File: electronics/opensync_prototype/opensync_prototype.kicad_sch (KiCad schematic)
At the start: 0 parts

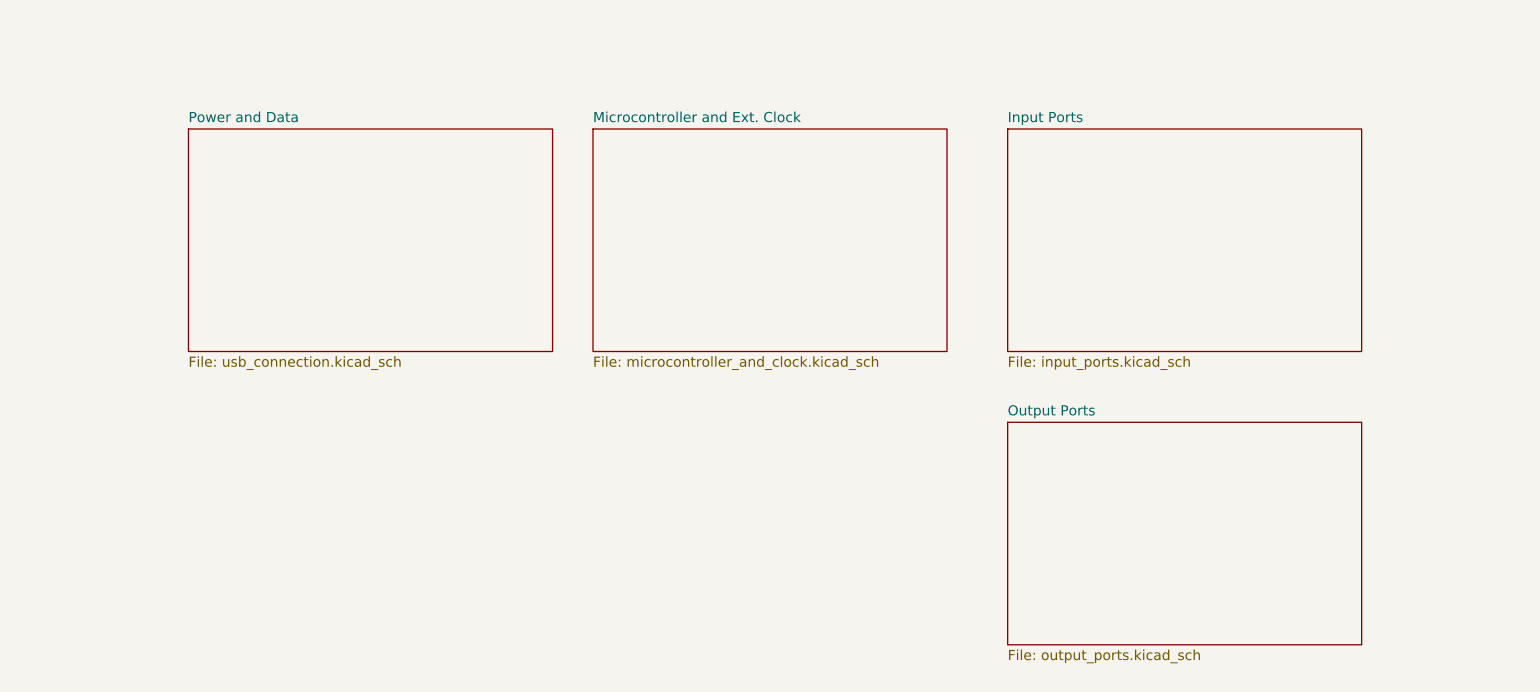
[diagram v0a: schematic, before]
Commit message: Emergency backup
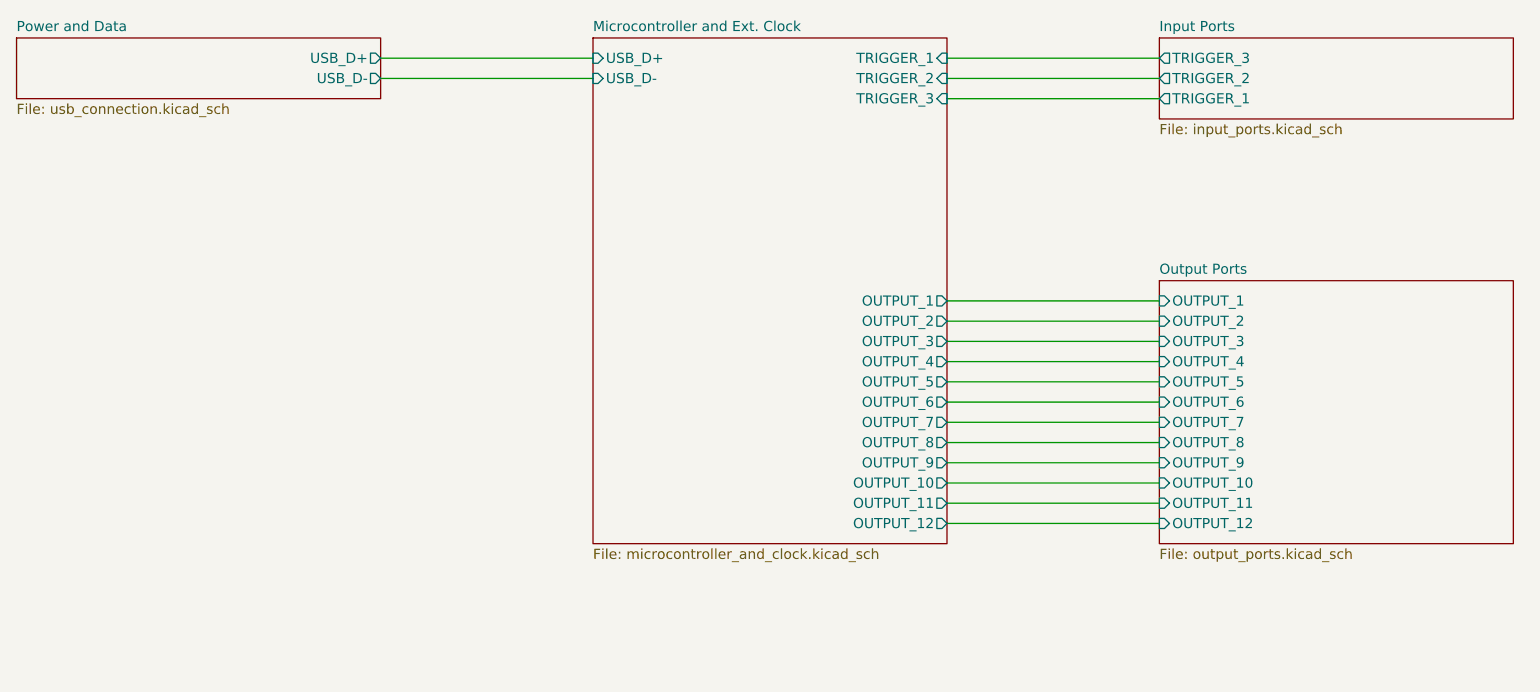
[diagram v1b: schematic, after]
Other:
- sheet Input Ports ports: added TRIGGER_1, TRIGGER_2, TRIGGER_3; removed none
- sheet Microcontroller and Ext. Clock ports: added OUTPUT_1, OUTPUT_10, OUTPUT_11, OUTPUT_12, OUTPUT_2, OUTPUT_3, OUTPUT_4, OUTPUT_5, OUTPUT_6, OUTPUT_7, OUTPUT_8, OUTPUT_9, TRIGGER_1, TRIGGER_2, TRIGGER_3, USB_D+, USB_D-; removed none
- sheet Output Ports ports: added OUTPUT_1, OUTPUT_10, OUTPUT_11, OUTPUT_12, OUTPUT_2, OUTPUT_3, OUTPUT_4, OUTPUT_5, OUTPUT_6, OUTPUT_7, OUTPUT_8, OUTPUT_9; removed none
- sheet Power and Data ports: added USB_D+, USB_D-; removed none

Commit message: Backup
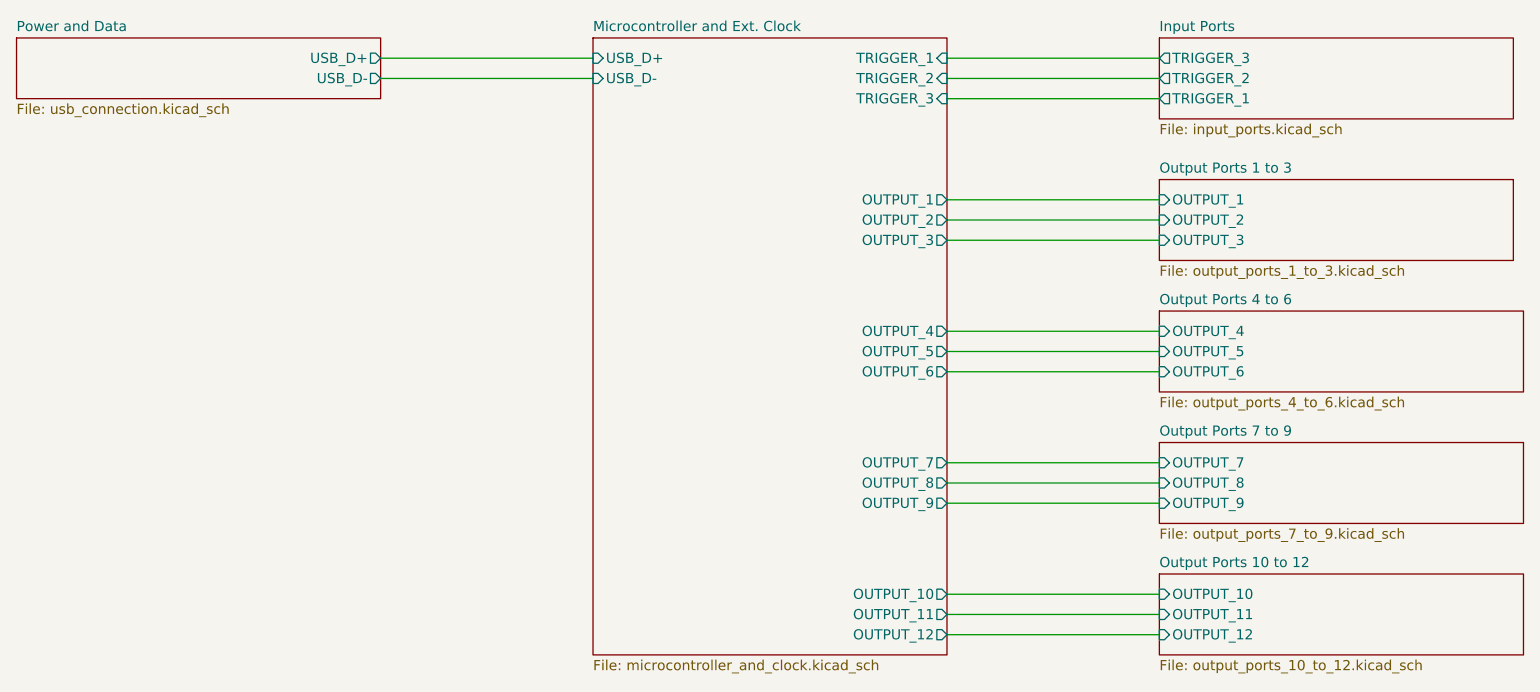
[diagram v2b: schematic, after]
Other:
- removed sheet Output Ports
- added sheet Output Ports 1 to 3 (output_ports_1_to_3.kicad_sch)
- added sheet Output Ports 10 to 12 (output_ports_10_to_12.kicad_sch)
- added sheet Output Ports 4 to 6 (output_ports_4_to_6.kicad_sch)
- added sheet Output Ports 7 to 9 (output_ports_7_to_9.kicad_sch)
